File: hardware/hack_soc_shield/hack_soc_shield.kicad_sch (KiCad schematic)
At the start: 29 parts, among them J1 Conn_01x05_Pin, J10 Conn_01x27_Female, J11 Conn_01x20_Female, J2 Conn_01x10_Pin, J3 Conn_01x06_Pin, J4 Conn_01x06_Pin, J5 Conn_01x05_Pin, SW1 SW_Push, SW2 SW_DIP_x02, U1 23LC1024, U2 23LC1024, U3 23LC1024

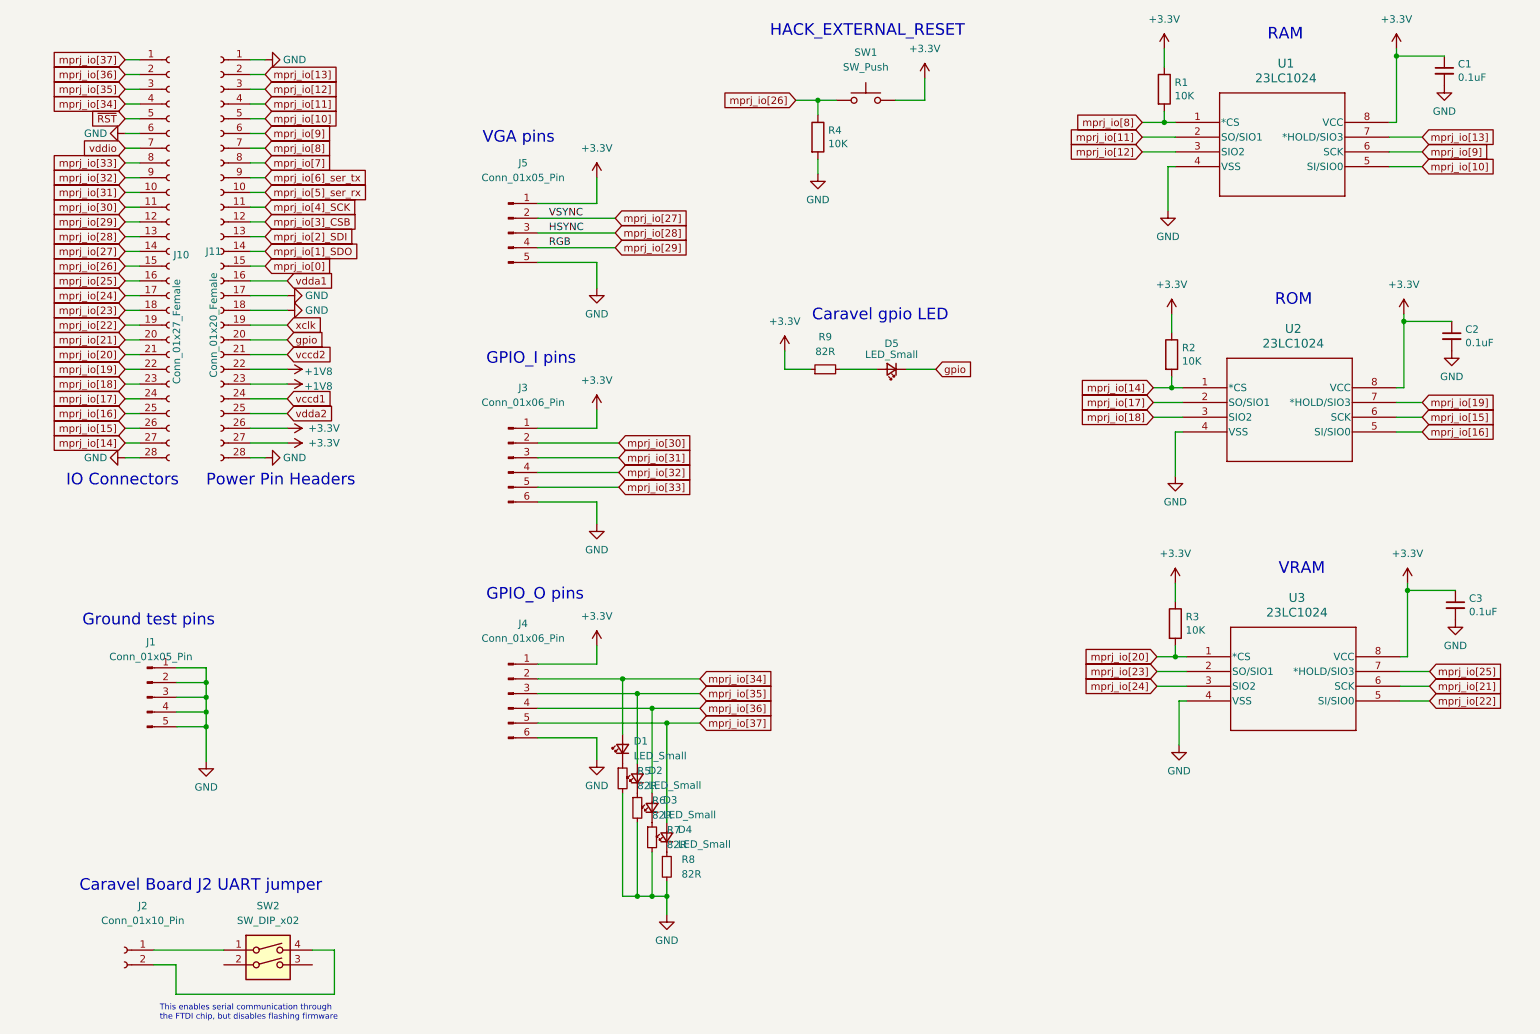
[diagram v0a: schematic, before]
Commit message: Update hack_soc_shield
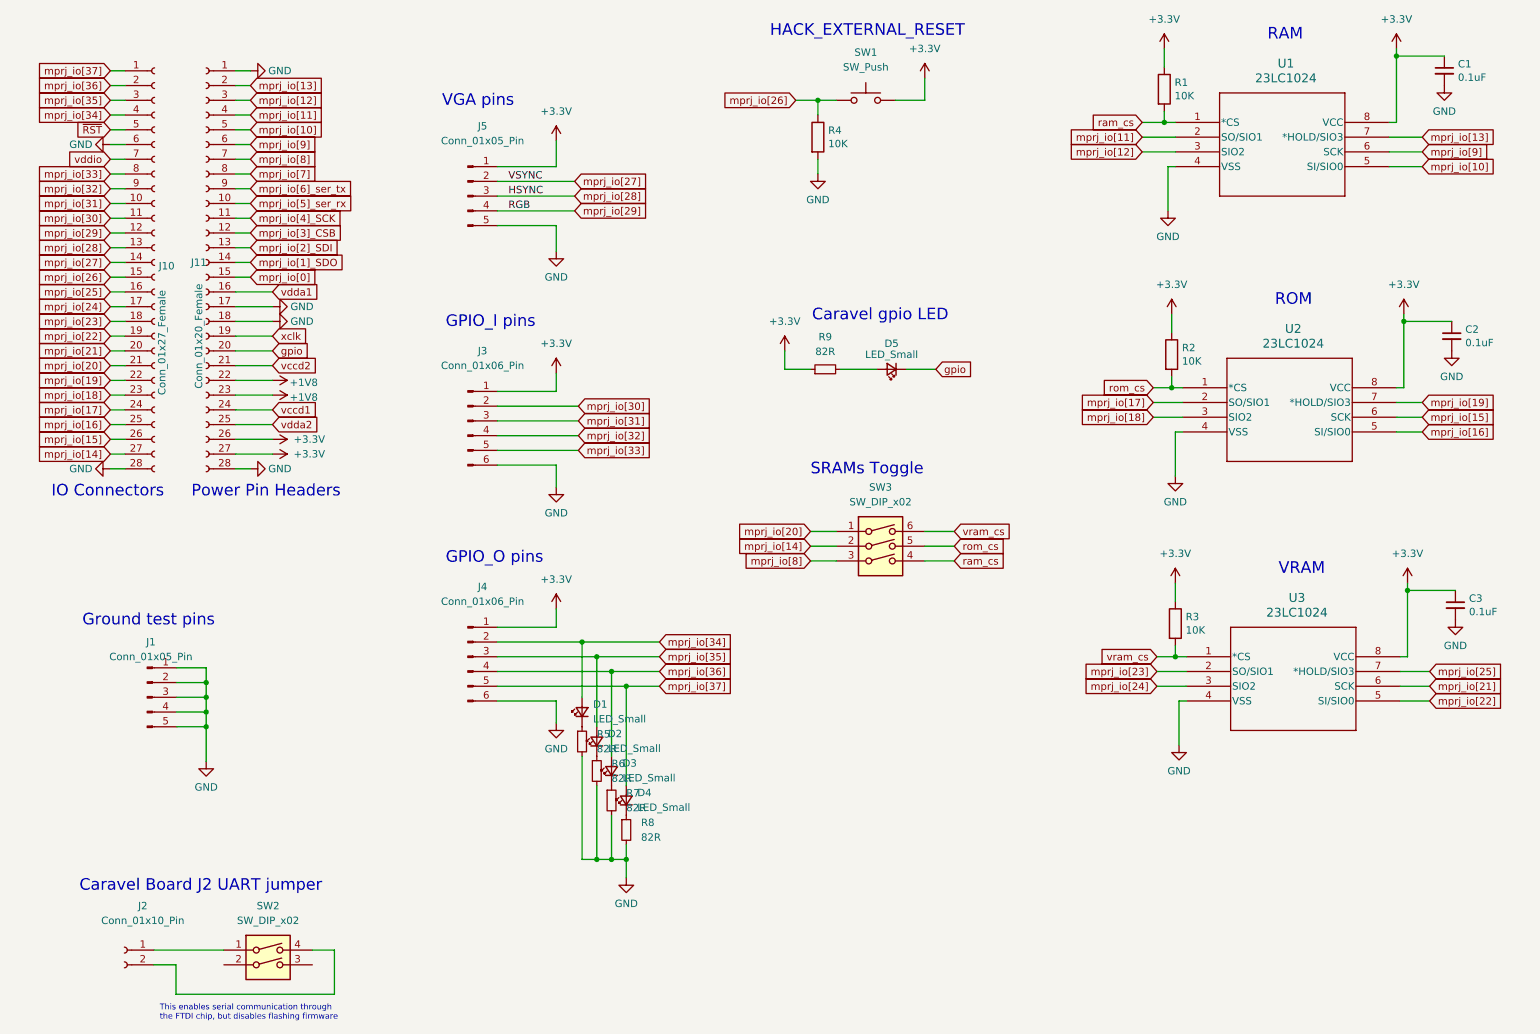
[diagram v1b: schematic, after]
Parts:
- added SW3: SW_DIP_x02, Button_Switch_THT:SW_DIP_SPSTx03_Slide_9.78x9.8mm_W7.62mm_P2.54mm, symbol Switch:SW_DIP_x03
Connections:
- net mprj_io[14]: now also SW3.2; no longer R2.2, U2.1 (*CS)
- net mprj_io[20]: now also SW3.1; no longer R3.2, U3.1 (*CS)
- net mprj_io[8]: now also SW3.3; no longer R1.2, U1.1 (*CS)
- new net ram_cs: R1.2, SW3.4, U1.1 (*CS)
- new net rom_cs: R2.2, SW3.5, U2.1 (*CS)
- new net vram_cs: R3.2, SW3.6, U3.1 (*CS)
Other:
- note added: "SRAMs Toggle"
- moved on the sheet: D1, D2, D3, D4, J10, J11, J3, J4, J5, R5, R6, R7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
